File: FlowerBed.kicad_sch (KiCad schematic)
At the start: 28 parts, among them J1 Conn_01x02, J2 AudioJack3_SwitchTR, J3 AudioJack3_SwitchTR, J4 Conn_01x07, J5 Conn_01x16, J6 Conn_01x02, SW0 SW_SPST, SW1 SW_SPST, SW2 SW_SPST, SW3 SW_SPST, SW4 SW_SPST, SW5 SW_SPST, SW6 SW_SPST, SW7 SW_SPST, U1 PAM8302AASCR

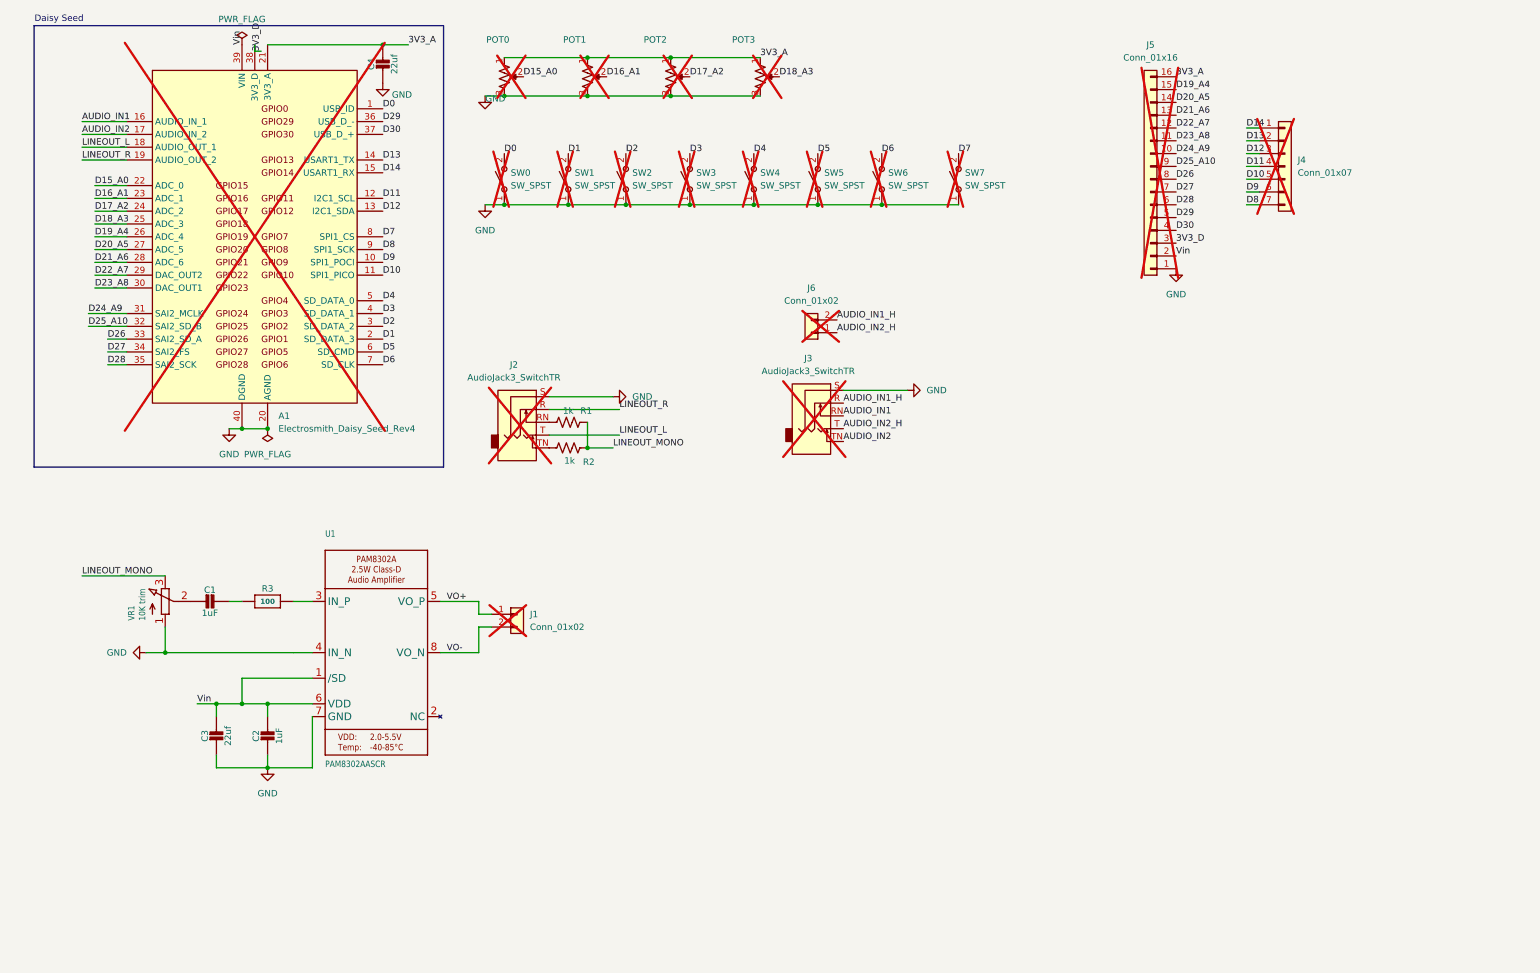
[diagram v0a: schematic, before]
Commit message: Legacy active sum
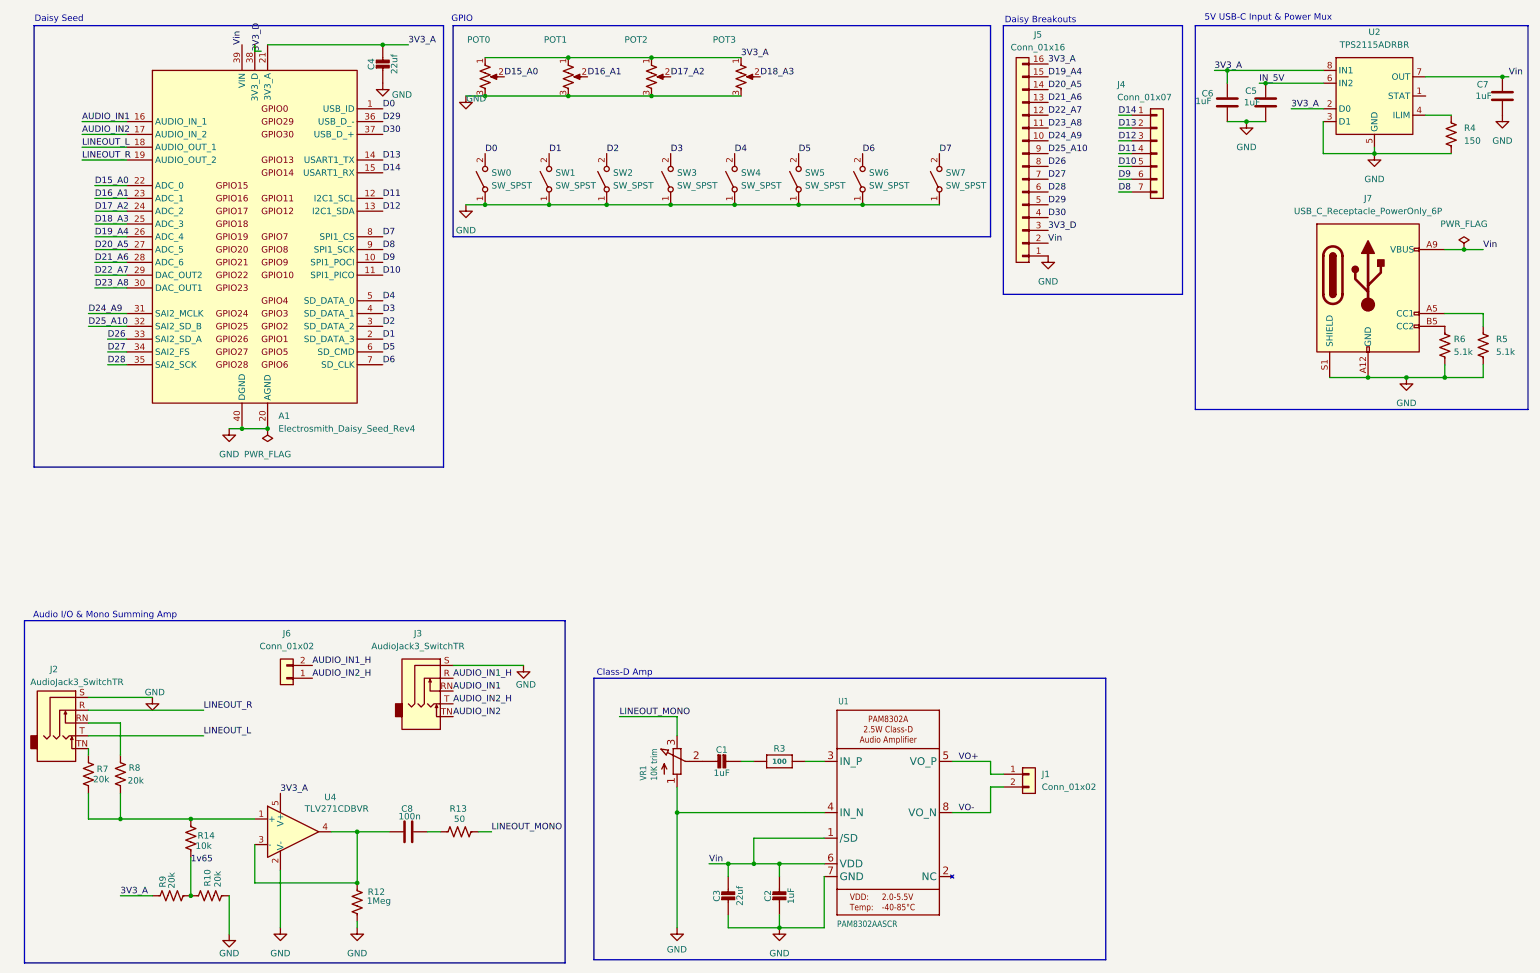
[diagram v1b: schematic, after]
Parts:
- removed R1, R2: 1k, Resistor_SMD:R_01005_0402Metric, symbol Device:R_US
- added C5, C6, C7: 1uF, symbol Device:C
- added C8: 100n, symbol Device:C
- added J7: USB_C_Receptacle_PowerOnly_6P, symbol Connector:USB_C_Receptacle_PowerOnly_6P
- added R10, R7, R8, R9: 20k, Resistor_SMD:R_01005_0402Metric, symbol Device:R_US
- added R12: 1Meg, Resistor_SMD:R_01005_0402Metric, symbol Device:R_US
- added R13: 50, Resistor_SMD:R_01005_0402Metric, symbol Device:R_US
- added R14: 10k, Resistor_SMD:R_01005_0402Metric, symbol Device:R_US
- added R4: 150, symbol Device:R_US
- added R5, R6: 5.1k, symbol Device:R_US
- added U2: TPS2115ADRBR, Package_TO_SOT_SMD:SOT-583-8, symbol Flowerbed:TPS2115ADRBR
- added U4: TLV271CDBVR, Package_TO_SOT_SMD:SOT-353_SC-70-5, symbol Amplifier_Operational:TLV172IDCK
- A1, J1, J2, J3, J4, J5, J6, POT0, POT1, POT2, POT3, SW0, SW1, SW2, SW3, SW4, SW5, SW6, SW7: now fitted
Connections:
- net 3V3_A: now also C6.1, R9.2, U2.2 (D0), U2.8 (IN1), U4.5 (V+)
- net GND: now also C5.2, C6.2, C7.2, J7.A12 (GND), J7.B12 (GND), J7.S1 (SHIELD), R10.1, R12.1, R4.2, R5.1, R6.1, U2.3 (D1), U2.5 (GND), U4.2 (V-)
- net LINEOUT_MONO: now also R13.1
- net Vin: now also C7.1, J7.A9 (VBUS), J7.B9 (VBUS), U2.7 (OUT)
- net at J2.RN: now also R8.2
- net at J2.TN: now also R7.2
- new net: C8.2, R13.2
- new net: R4.1, U2.4 (ILIM)
- new net: R14.2, R7.1, R8.1, U4.1 (+)
- new net: C8.1, R12.2, U4.3 (-), U4.4
- new net: J7.A5 (CC1), R5.2
- new net: J7.B5 (CC2), R6.2
- new net 1v65: R10.2, R14.1, R9.1
- new net IN_5V: C5.1, U2.6 (IN2)
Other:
- note added: "5V USB-C Input & Power Mux"
- note added: "Audio I/O & Mono Summing Amp"
- note added: "Class-D Amp"
- note added: "Daisy Breakouts"
- note added: "GPIO"
- moved on the sheet: C1, C2, C3, R3, U1, VR1
